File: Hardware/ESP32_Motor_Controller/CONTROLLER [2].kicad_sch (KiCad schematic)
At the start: 19 parts, among them SW1 TS-1088-AR02016, SW2 TS-1088-AR02016

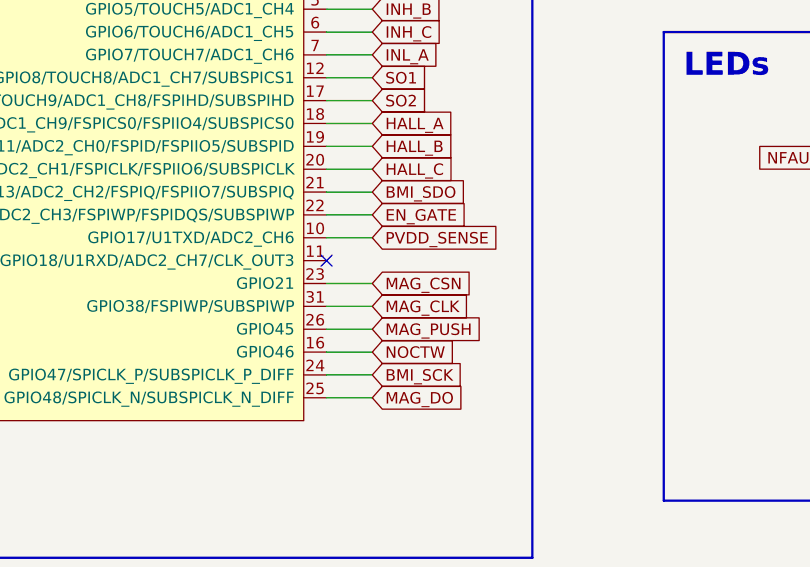
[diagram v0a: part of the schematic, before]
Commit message: PCB Layout Update
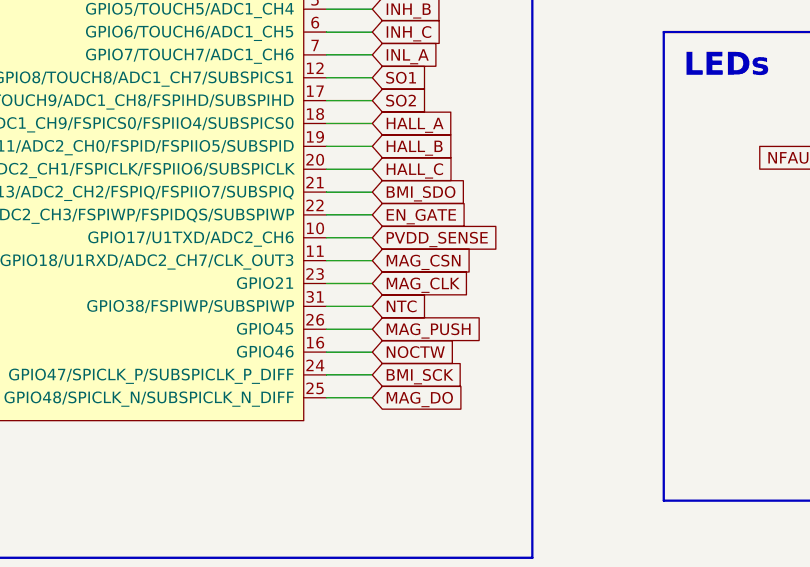
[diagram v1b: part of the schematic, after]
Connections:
- net MAG_CLK: now also MCU1.23 (GPIO21); no longer MCU1.31 (GPIO38/FSPIWP/SUBSPIWP)
- net MAG_CSN: now also MCU1.11 (GPIO18/U1RXD/ADC2_CH7/CLK_OUT3); no longer MCU1.23 (GPIO21)
- new net NTC: MCU1.31 (GPIO38/FSPIWP/SUBSPIWP)
- no-connect marks 1 -> 0

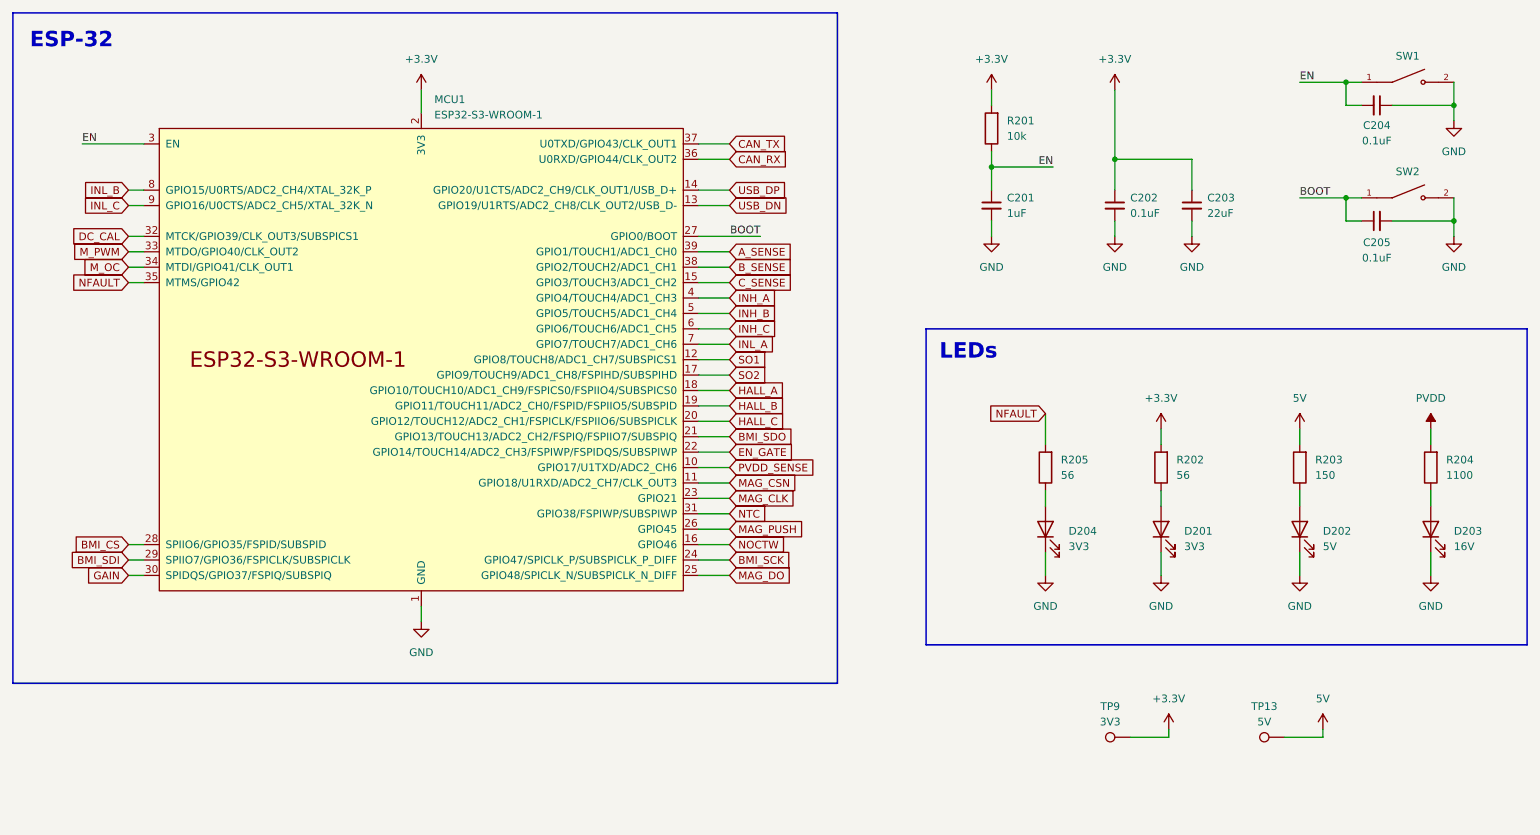
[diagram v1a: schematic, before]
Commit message: Finished Layout V1
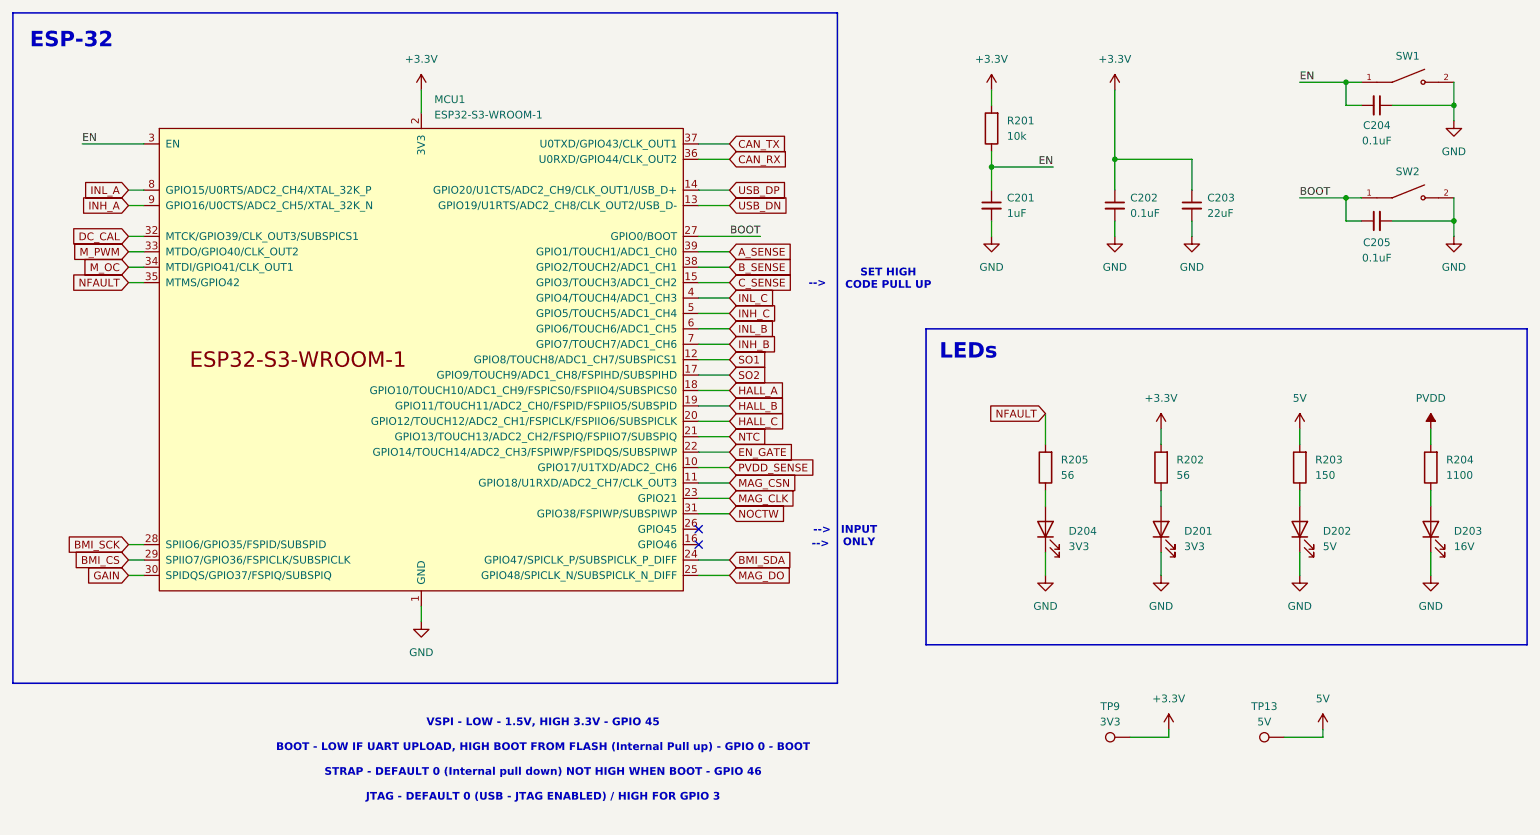
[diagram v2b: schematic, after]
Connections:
- net BMI_SDI is gone; now on net BMI_CS: MCU1.29 (SPIIO7/GPIO36/FSPICLK/SUBSPICLK)
- net BMI_SDO is gone; now on net NTC: MCU1.21 (GPIO13/TOUCH13/ADC2_CH2/FSPIQ/FSPIIO7/SUBSPIQ)
- net BMI_CS: no longer MCU1.28 (SPIIO6/GPIO35/FSPID/SUBSPID)
- net BMI_SCK: now also MCU1.28 (SPIIO6/GPIO35/FSPID/SUBSPID); no longer MCU1.24 (GPIO47/SPICLK_P/SUBSPICLK_P_DIFF)
- net INH_A: now also MCU1.9 (GPIO16/U0CTS/ADC2_CH5/XTAL_32K_N); no longer MCU1.4 (GPIO4/TOUCH4/ADC1_CH3)
- net INH_B: now also MCU1.7 (GPIO7/TOUCH7/ADC1_CH6); no longer MCU1.5 (GPIO5/TOUCH5/ADC1_CH4)
- net INH_C: now also MCU1.5 (GPIO5/TOUCH5/ADC1_CH4); no longer MCU1.6 (GPIO6/TOUCH6/ADC1_CH5)
- net INL_A: now also MCU1.8 (GPIO15/U0RTS/ADC2_CH4/XTAL_32K_P); no longer MCU1.7 (GPIO7/TOUCH7/ADC1_CH6)
- net INL_B: now also MCU1.6 (GPIO6/TOUCH6/ADC1_CH5); no longer MCU1.8 (GPIO15/U0RTS/ADC2_CH4/XTAL_32K_P)
- net INL_C: now also MCU1.4 (GPIO4/TOUCH4/ADC1_CH3); no longer MCU1.9 (GPIO16/U0CTS/ADC2_CH5/XTAL_32K_N)
- net NOCTW: now also MCU1.31 (GPIO38/FSPIWP/SUBSPIWP); no longer MCU1.16 (GPIO46)
- net NTC: no longer MCU1.31 (GPIO38/FSPIWP/SUBSPIWP)
- net MAG_PUSH: no longer names the net of MCU1.26 (GPIO45)
- new net BMI_SDA: MCU1.24 (GPIO47/SPICLK_P/SUBSPICLK_P_DIFF)
- no-connect marks 0 -> 2
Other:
- note added: "-->"
- note added: "INPUT ONLY"
- note added: "SET HIGH CODE PULL UP"
- note added: "VSPI - LOW - 1.5V, HIGH 3.3V - GPIO 45 BOOT - LOW IF UART UPLOAD, HIGH BOOT FROM FLASH (Internal Pull up) - GPIO 0 - BOOT STRAP - DEFAULT 0 (Internal pull down) NOT HIGH WHEN BOOT - GPIO 46 JTAG - DEFAULT 0 (USB - JTAG ENABLED) / HIGH FOR GPIO 3"

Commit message: PCB_V2
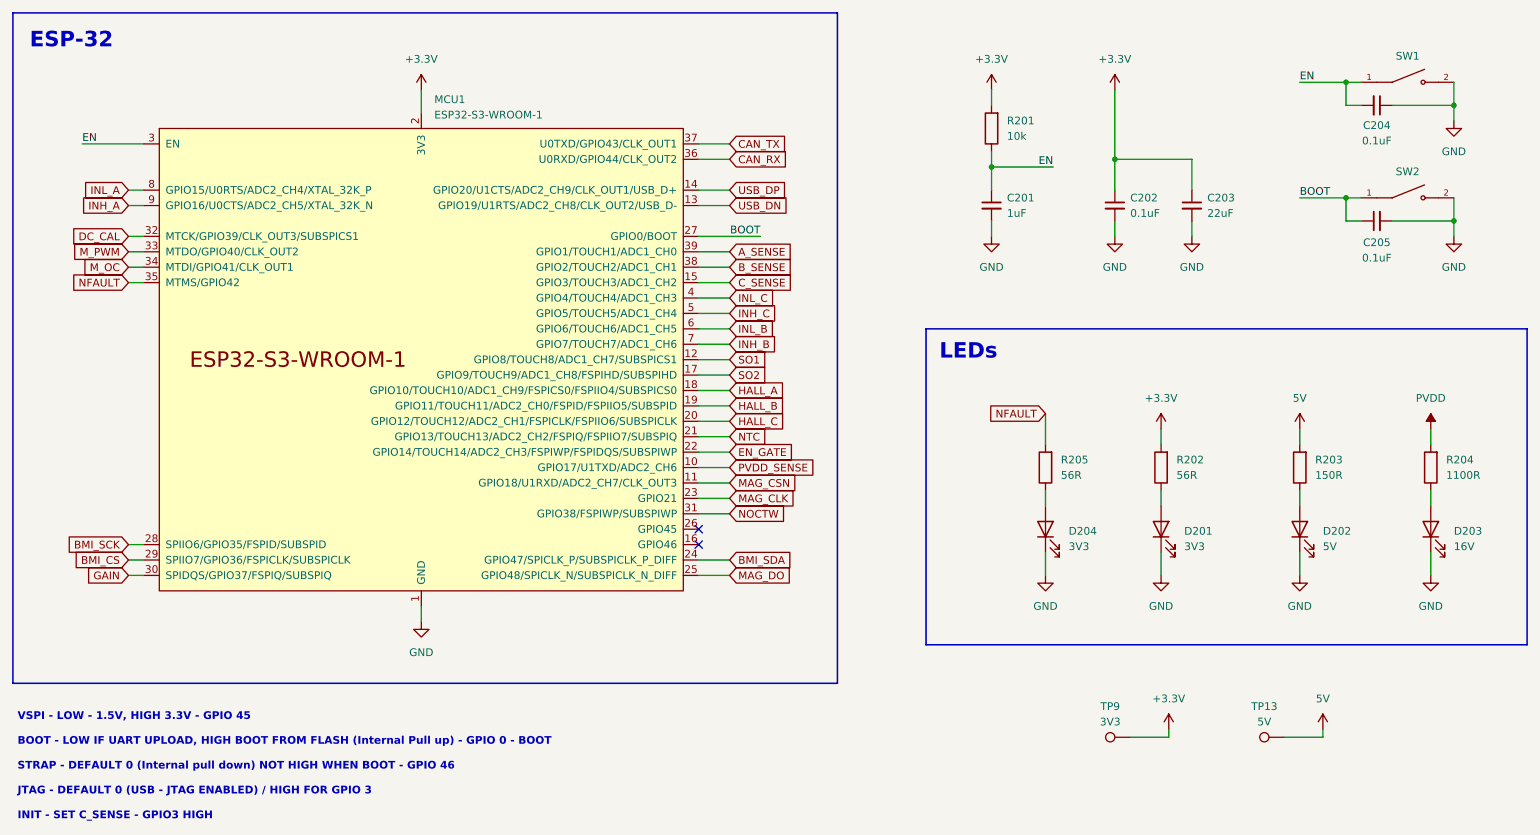
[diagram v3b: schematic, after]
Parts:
- C201: footprint Capacitor_SMD:C_0402_1005Metric -> Capacitor_SMD:C_0603_1608Metric
- C203: footprint Capacitor_SMD:C_0402_1005Metric -> Capacitor_SMD:C_0805_2012Metric
- R202, R205: value 56 -> 56R
- R203: value 150 -> 150R
- R204: value 1100 -> 1100R
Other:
- note added: "VSPI - LOW - 1.5V, HIGH 3.3V - GPIO 45 BOOT - LOW IF UART UPLOAD, HIGH BOOT FROM FLASH (Internal Pull up) - GPIO 0 - BOOT STRAP - DEFAULT 0 (Internal pull down) NOT HIGH WHEN BOOT - GPIO 46 JTAG - DEFAULT 0 (USB - JTAG ENABLED) / HIGH FOR GPIO 3 INIT - SET C_SENSE - GPIO3 HIGH"
- note removed: "-->"
- note removed: "INPUT ONLY"
- note removed: "SET HIGH CODE PULL UP"
- note removed: "VSPI - LOW - 1.5V, HIGH 3.3V - GPIO 45 BOOT - LOW IF UART UPLOAD, HIGH BOOT FROM FLASH (Internal Pull up) - GPIO 0 - BOOT STRAP - DEFAULT 0 (Internal pull down) NOT HIGH WHEN BOOT - GPIO 46 JTAG - DEFAULT 0 (USB - JTAG ENABLED) / HIGH FOR GPIO 3"
- company: (none) -> ANGEL PELEGRY VELASCO
